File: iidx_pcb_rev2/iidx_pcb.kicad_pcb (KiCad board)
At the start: 2 copper layers, 68.6 x 64.1 mm, 7 parts, among them J2 Conn_01x05, J3 Conn_01x12, U1 RP2040-Zero

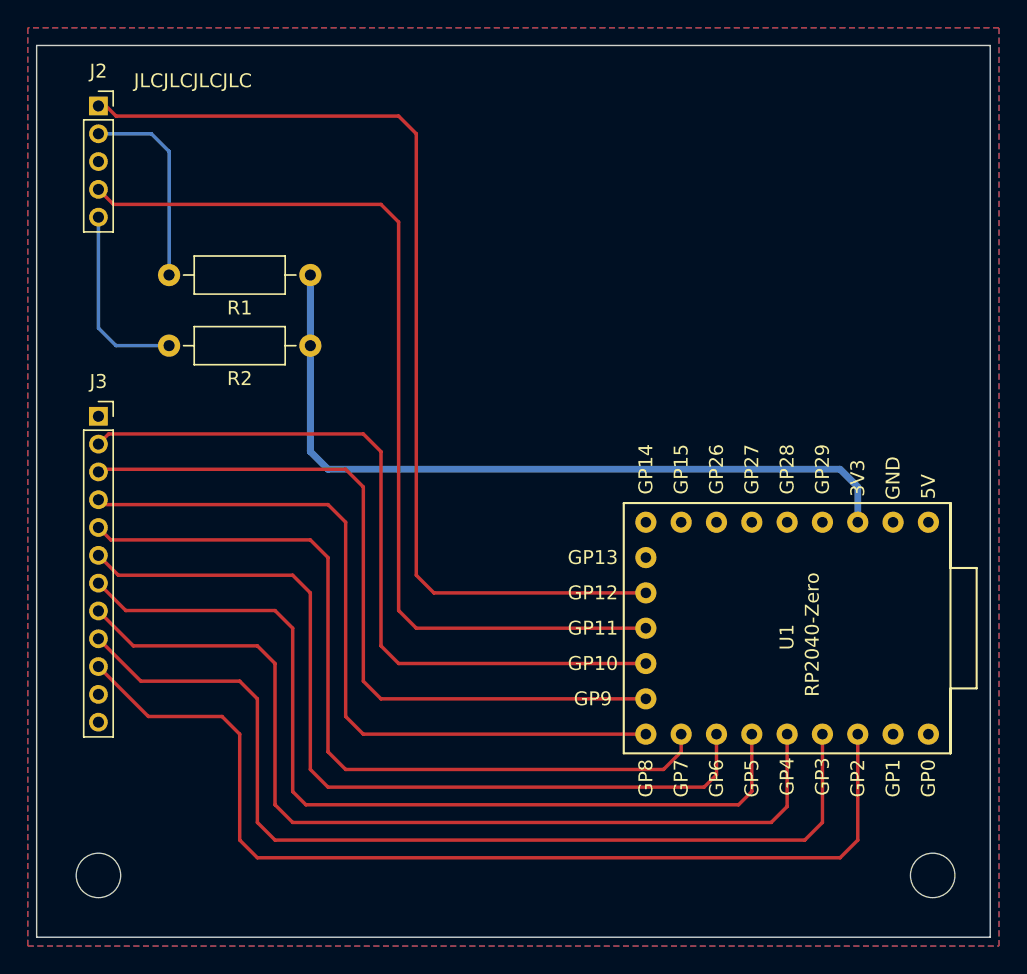
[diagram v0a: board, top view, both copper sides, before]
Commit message: update iidx_pcb_rev2
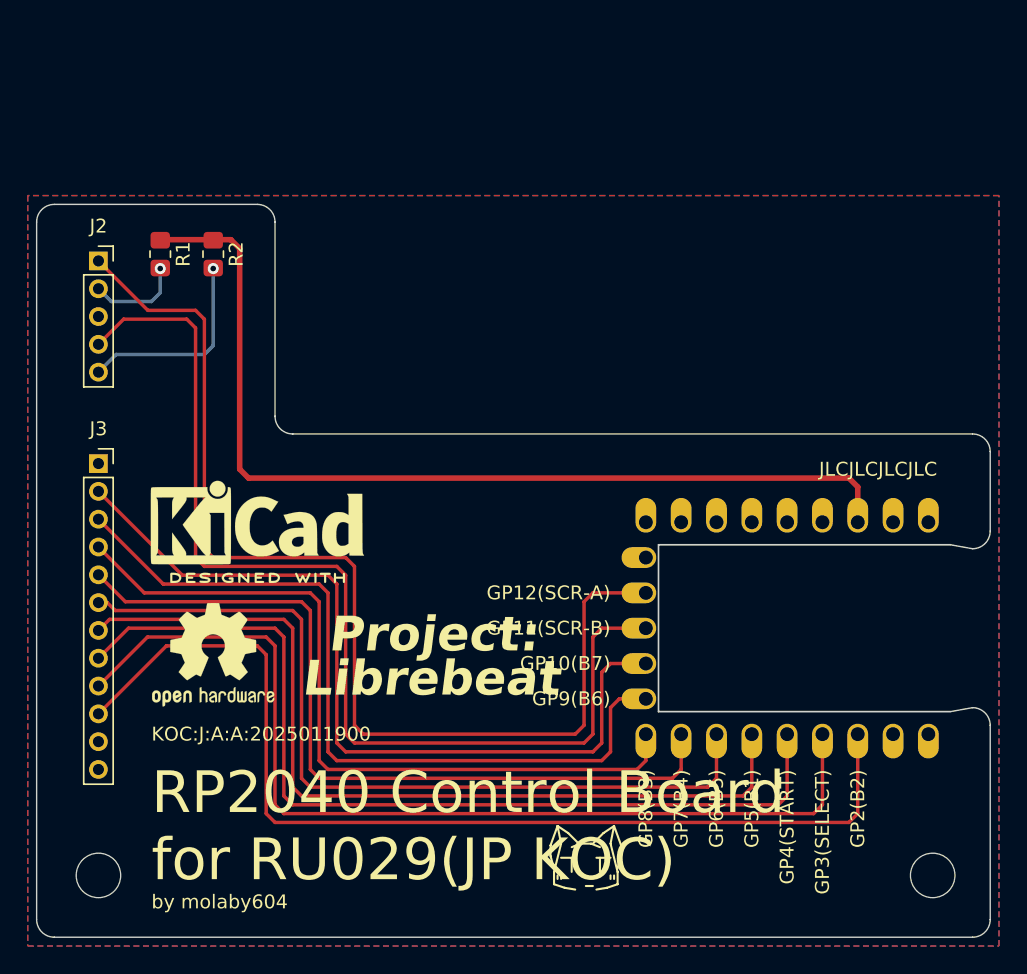
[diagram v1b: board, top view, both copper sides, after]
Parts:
- removed U1: RP2040-Zero, rp2040:RP2040-Zero
- added S1: OSHW_Logo, Symbol:OSHW-Logo2_9.8x8mm_SilkScreen, F.Cu at (59.1, 131.4)
- added S2: KiCad_Logo, Symbol:KiCad-Logo2_6mm_SilkScreen, F.Cu at (62.2, 121.9)
- added U2: rp2040-zero, mcu:rp2040-zero-tht, F.Cu at (100.3, 129.5)
- R1, R2: footprint Resistor_THT:R_Axial_DIN0207_L6.3mm_D2.5mm_P10.16mm_Horizontal -> Resistor_SMD:R_0805_2012Metric_Pad1.20x1.40mm_HandSolder
- moved J2 11.1 mm to (50.8, 103.1)
- moved R1 10.9 mm to (55.2, 102.6), turned to -90 degrees
- moved R2 9.60 mm to (59.1, 102.6), turned to -90 degrees
- moved J3 3.40 mm to (50.8, 117.7)
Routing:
- net 3V3: track 55.7 -> 69.4 mm
- net SCR_LEDA: track 14.5 -> 6.82 mm, vias 0 -> 1
- net SCR_TRCB: track 69.1 -> 76.6 mm
- net SCR_TRCA: track 72.5 -> 79.3 mm
- net KEY_7: track 54.7 -> 59.4 mm
- net KEY_6: track 54.5 -> 57.0 mm
- net KEY_5: track 62.1 -> 60.1 mm
- net KEY_2: track 72.9 -> 74.6 mm
- net KEY_1: track 65.0 -> 63.3 mm
- net KEY_4: track 59.1 -> 57.5 mm
- net SCR_LEDB: track 13.6 -> 14.6 mm, vias 0 -> 1
- net KEY_SEL: track 70.2 -> 70.8 mm
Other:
- board size 68.6 x 64.1 mm -> 68.6 x 52.7 mm
- board text added: "GP10(B7)"
- board text added: "GP11(SCR-B)"
- board text added: "GP12(SCR-A)"
- board text added: "GP2(B2)"
- board text added: "GP3(SELECT)"
- board text added: "GP4(START)"
- board text added: "GP5(B1)"
- board text added: "GP6(B5)"
- board text added: "GP7(B4)"
- board text added: "GP8(B3)"
- board text added: "GP9(B6)"
- board text added: "KOC:J:A:A:2025011900"
- board text added: "Librebeat"
- board text added: "Project:"
- board text added: "RP2040 Control Board for RU029(JP KOC)"
- board text added: "by molaby604"
- board text removed: "GP3"
- board text removed: "GP4"
